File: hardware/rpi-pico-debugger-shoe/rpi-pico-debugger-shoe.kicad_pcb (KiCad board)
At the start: 2 copper layers, 21 x 54.5 mm, 49 parts, among them J1 10118193-0001LF, J2 Conn_01x02, J3 Conn_01x03, J4 Conn_01x18, J5 Conn_01x20, J6 Conn_01x03, J7 Conn_01x03, J8 Conn_01x02, SW1 PTS810_SJK_250_SMTR_LFS, U1 RP2040, U2 AP2112K-3.3TRG1, U3 W25Q16JVSSIQ, Y1 12MHz

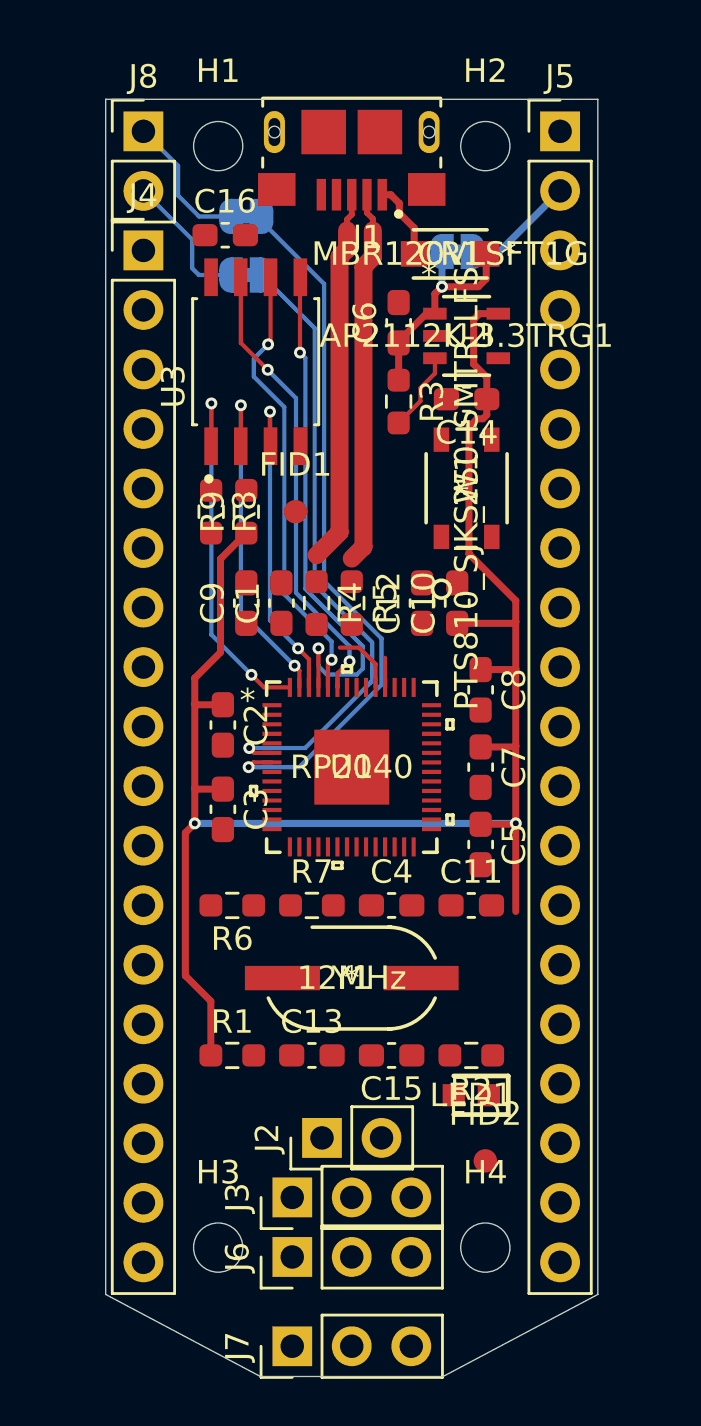
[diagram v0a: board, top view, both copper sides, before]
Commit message: Finished layout for v01
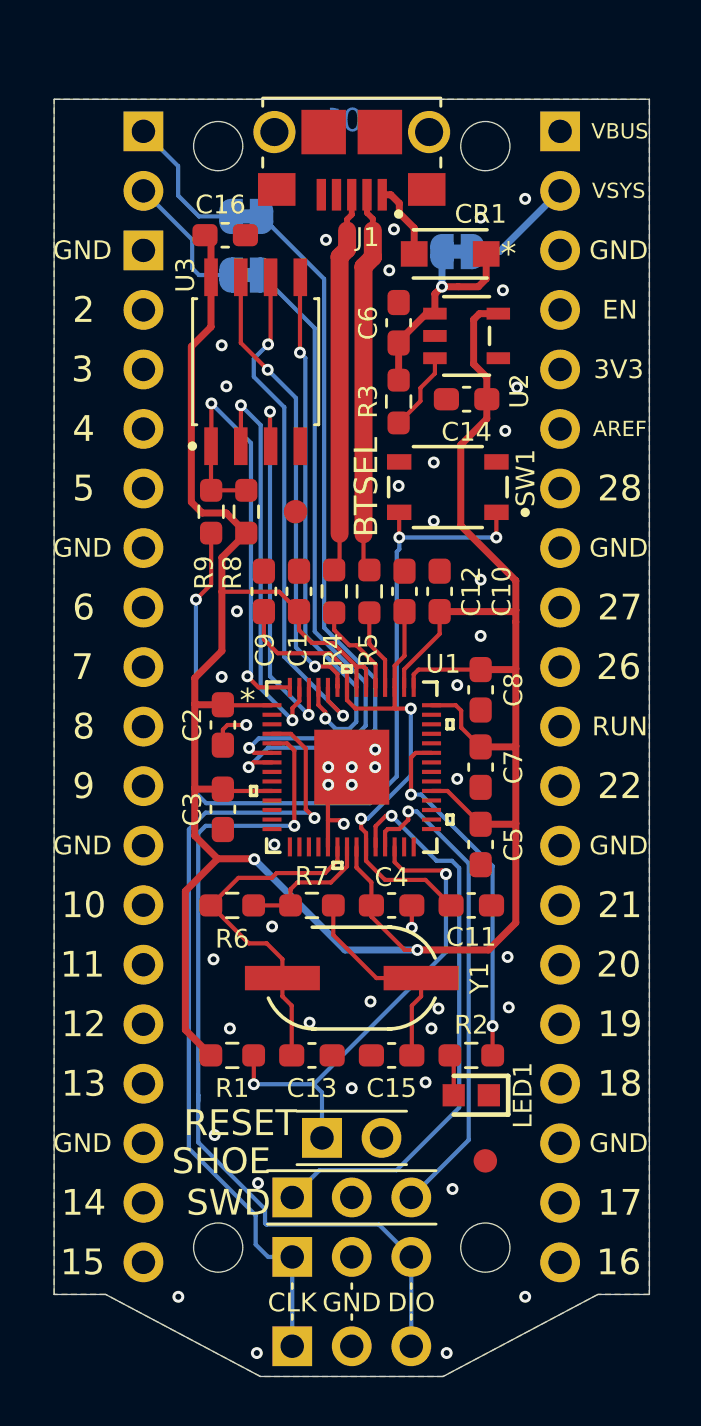
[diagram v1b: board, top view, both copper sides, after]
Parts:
- J1: footprint 10118193-0001LF:FCI_10118193-0001LF -> 10118193-0001LF:FCI_10118193-0001LF_no-slot
- J2, J8: footprint Connector_PinHeader_2.54mm:PinHeader_1x02_P2.54mm_Vertical -> custom:PinHeader_1x02_P2.54mm_Vertical_no-silk
- J3, J6, J7: footprint Connector_PinHeader_2.54mm:PinHeader_1x03_P2.54mm_Vertical -> custom:PinHeader_1x03_P2.54mm_Vertical_no-silk
- J4: footprint Connector_PinHeader_2.54mm:PinHeader_1x18_P2.54mm_Vertical -> custom:PinHeader_1x18_P2.54mm_Vertical_no-silk
- J5: footprint Connector_PinHeader_2.54mm:PinHeader_1x20_P2.54mm_Vertical -> custom:PinHeader_1x20_P2.54mm_Vertical_no-silk
- moved C1 0.90 mm to (135.2, 97.0)
- moved C10 0.90 mm to (141.2, 97.0)
- moved C12 0.90 mm to (139.8, 97.0)
- moved C9 0.90 mm to (133.8, 97.0)
- moved R4 0.90 mm to (136.8, 97.0)
- moved R5 0.90 mm to (138.2, 97.0)
- moved SW1 0.80 mm to (141.6, 92.5), turned to 180 degrees
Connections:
- J5 pad 8: Net-(J5-Pad8) -> GND
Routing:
- net +3V3: track 75.0 -> 126.0 mm
- net /TARGET_SWDIO: track 0.00 -> 37.3 mm, vias 0 -> 1
- net /USB_BOOT: track 0.00 -> 37.1 mm, vias 0 -> 3
- net /TARGET_SWCLK: track 0.00 -> 35.1 mm, vias 0 -> 1
- net /+1.1V: track 0.00 -> 25.8 mm, vias 0 -> 2
- net /SWCLK: track 0.00 -> 24.5 mm, vias 0 -> 1
- net /SWDIO: track 0.00 -> 21.0 mm, vias 0 -> 1
- net /RUN: track 0.00 -> 20.6 mm, vias 0 -> 2
- net /GPIO25: track 0.00 -> 15.4 mm, vias 0 -> 2
- net /XIN: track 0.00 -> 15.1 mm
- net Net-(C15-Pad1): track 0.00 -> 9.23 mm
- net GND: track 0.00 -> 7.47 mm, vias 0 -> 47
- net /XOUT: track 0.00 -> 5.91 mm
- net /QSPI_CS: track 16.0 -> 19.6 mm
- net /QSPI_SCK: track 19.2 -> 22.1 mm
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- added copper zone on B.Cu, net GND
- added copper zone on F.Cu, net GND
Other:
- board size 21 x 54.5 mm -> 25.4 x 54.5 mm
- rule pad_to_mask_clearance: 0.0508 -> 0
- board text added: "10"
- board text added: "11"
- board text added: "12"
- board text added: "13"
- board text added: "14"
- board text added: "15"
- board text added: "16"
- board text added: "17"
- board text added: "18"
- board text added: "19"
- board text added: "2"
- board text added: "20"
- board text added: "21"
- board text added: "22"
- board text added: "26"
- board text added: "27"
- board text added: "28"
- board text added: "3"
- board text added: "3V3"
- board text added: "4"
- board text added: "5"
- board text added: "6"
- board text added: "7"
- board text added: "8"
- board text added: "9"
- board text added: "AREF"
- board text added: "BTSEL"
- board text added: "CLK"
- board text added: "DIO"
- board text added: "EN"
- board text added: "GND"
- board text added: "RESET"
- board text added: "RPi Pico Debugger Shoe"
- board text added: "RUN"
- board text added: "SHOE SWD"
- board text added: "TGT_RX"
- board text added: "TGT_TX"
- board text added: "VBUS"
- board text added: "VSYS"
- board text added: "v01"
